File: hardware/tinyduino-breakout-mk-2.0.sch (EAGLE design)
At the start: 5 parts, among them J1 DF12-32-DP

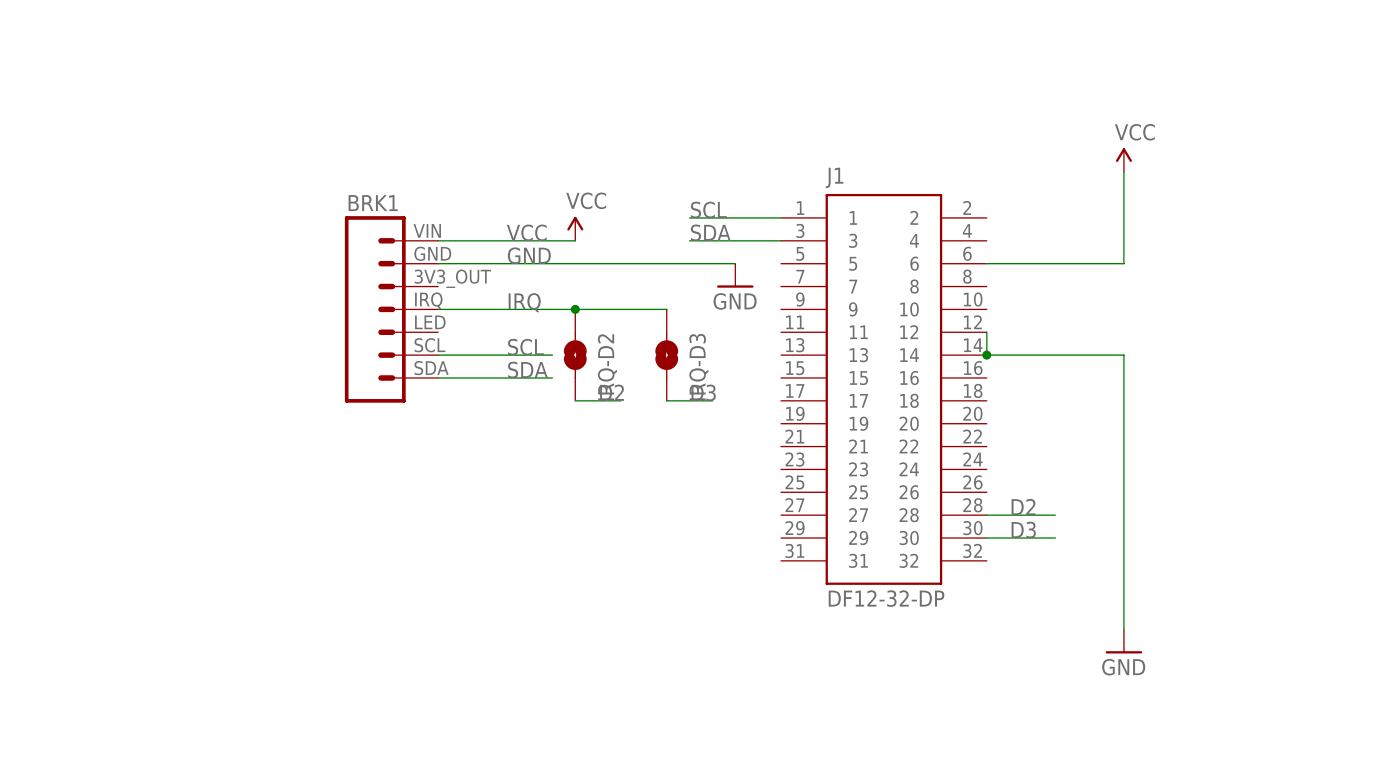
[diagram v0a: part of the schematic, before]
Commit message: tiny breakout attempt
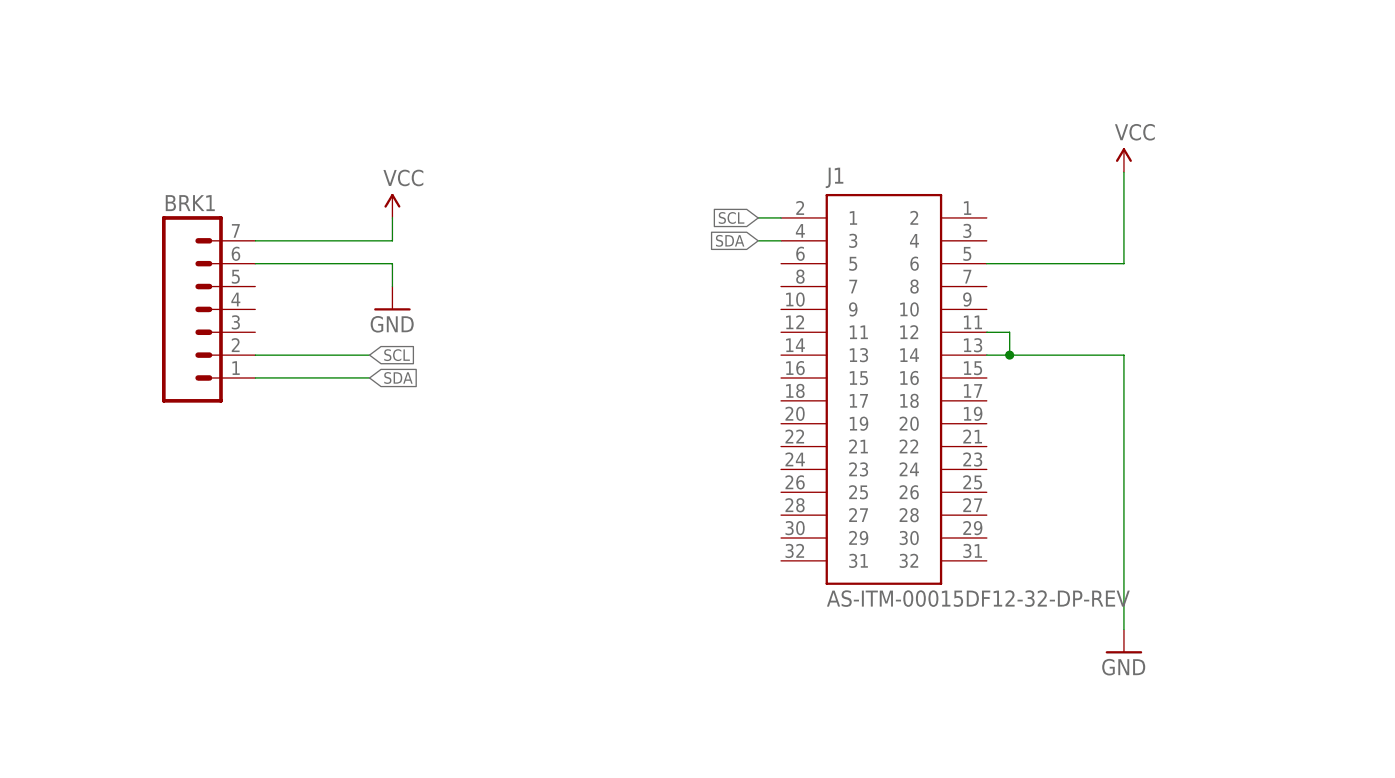
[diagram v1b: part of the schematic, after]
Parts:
- removed IRQ-D2, IRQ-D3: JUMPER-PAD-2-NOYES_SILK, A_butts:JUMPER-PAD-2-NOYES_SILK
- BRK1: value ADAFRUIT-SI1145-BREAKOUT -> ADAFRUIT-SI1145-BREAKOUTSMD-RA; device A_butts:ADAFRUIT-SI1145-BREAKOUT -> A_butts:ADAFRUIT-SI1145-BREAKOUTSMD-RA
- J1: value DF12-32-DP -> AS-ITM-00015DF12-32-DP-REV; device A_butts:AS-ITM-00015 -> A_butts:AS-ITM-00015DF12-32-DP-REV
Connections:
- removed net D2: IRQ-D2.2, J1.28
- removed net D3: IRQ-D3.2, J1.30
- removed net IRQ: BRK1.IRQ, IRQ-D2.1, IRQ-D3.1
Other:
- moved on the sheet: BRK1
